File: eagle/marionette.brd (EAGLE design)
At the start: 112.4 x 152.7 mm, 45 parts, among them J2 SWD_CONNECTOR, J3 2X10FE, J4 2X10FE, J5 2X10FE, J6 2X10FE, J7 2X10FE, U1 USB3318, U2 NCP705, U3 XCL206B, X1 ABS25-32.768KHZ-6-T

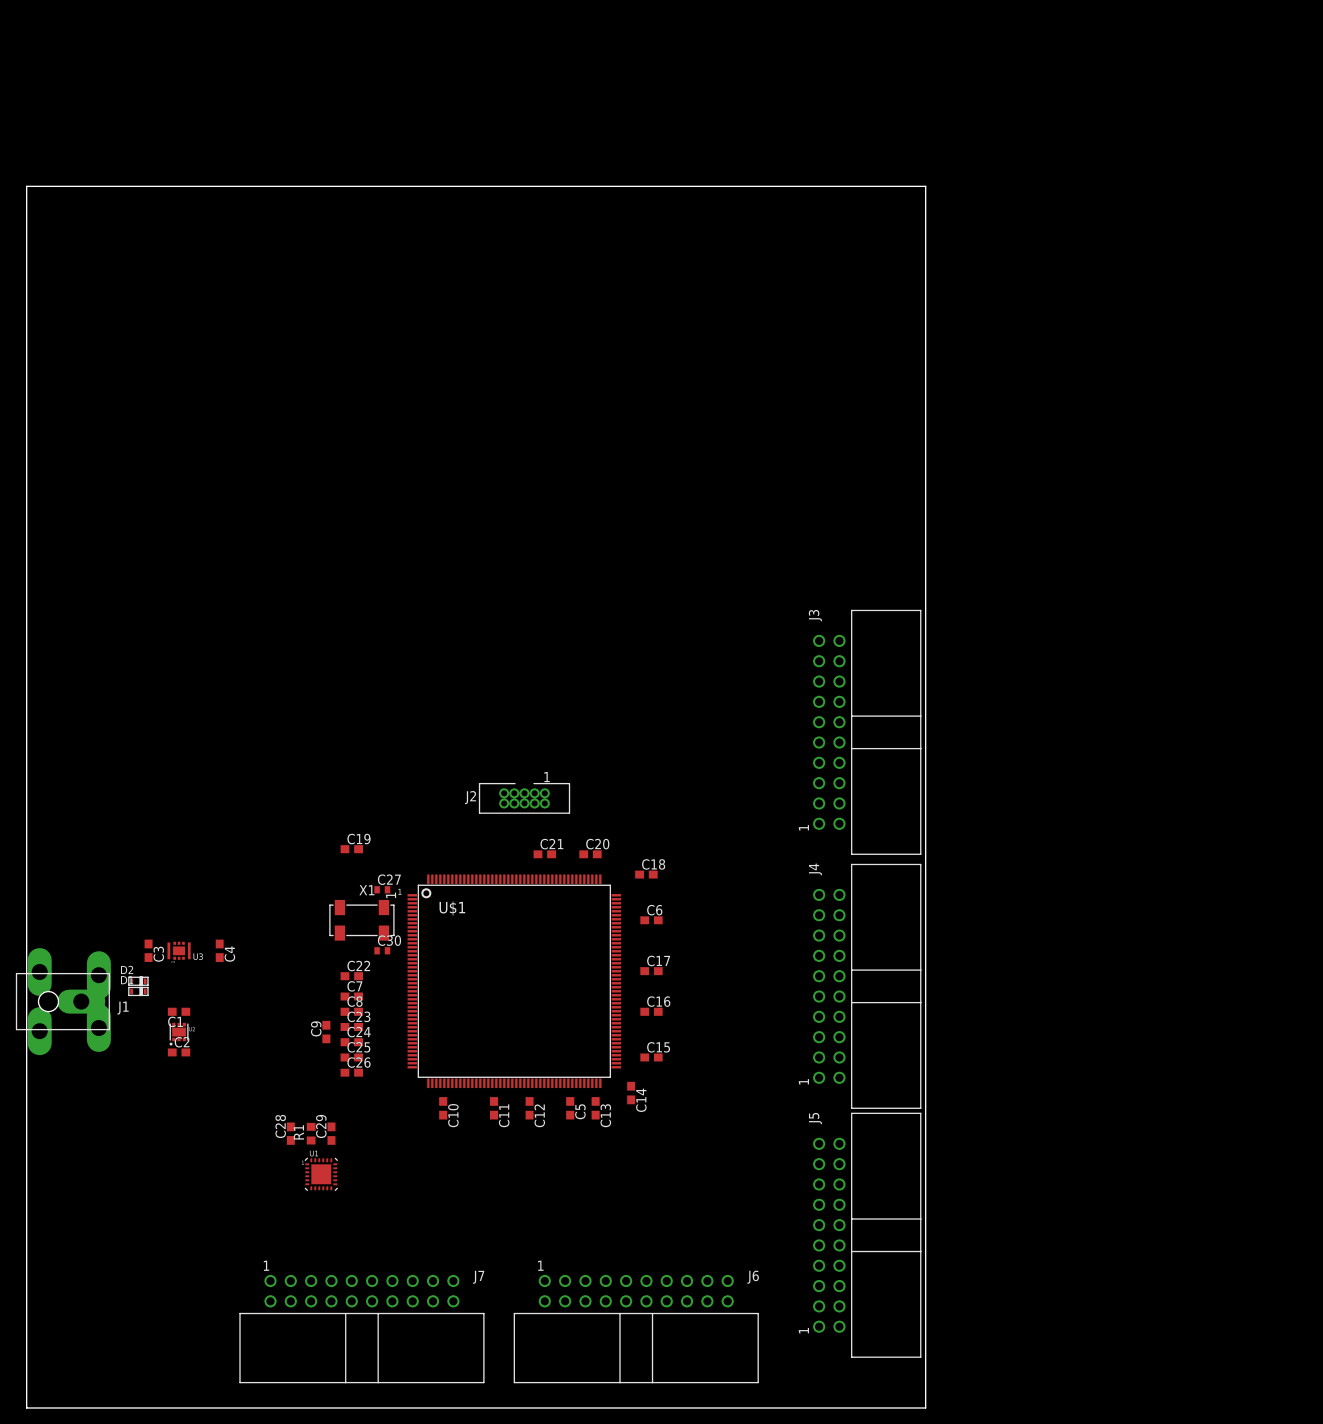
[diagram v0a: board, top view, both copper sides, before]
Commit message: Added connections to the EDGE CONNECTOR OF DEATH!!!!!!!!!!!!!
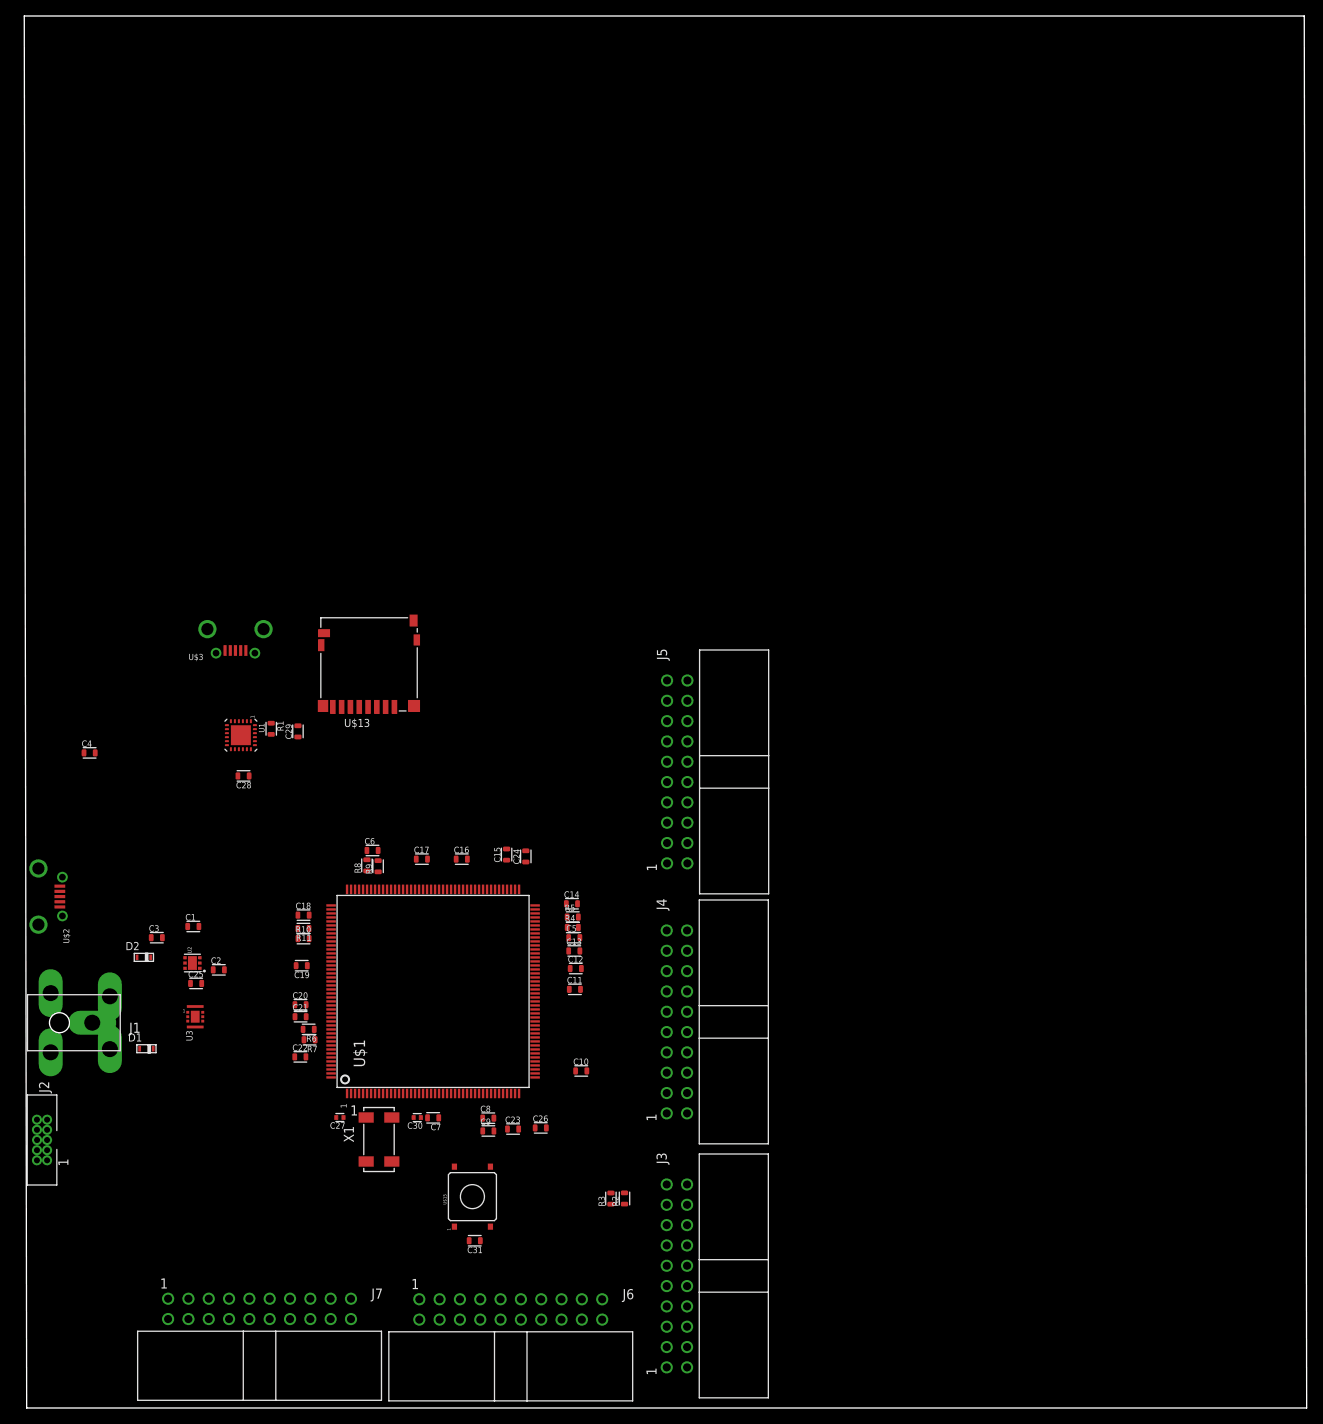
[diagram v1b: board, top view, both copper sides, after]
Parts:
- added C31: 100nF, 10V, rcl_custom:.0603-C
- added R10, R11, R2, R3, R4, R5, R6, R7, R8, R9: 4.7k, rcl_custom:.0603-C
- added U$13: CON_HIROSE_DM3D(MICROSD), con-microsd-hirose-dm3:HIROSE_DM3D(MICRO-SD)
- added U$15: PTS645, PTS645:SMT
- added U$2, U$3: ZX62D-B-5P8, con-hirose-microusb:ZX62D-B-5P8
- C1, C10, C11, C12, C13, C14, C15, C16, C17, C18, C19, C2, C20, C21, C22, C23, C24, C25, C26, C28, C29, C3, C4, C5, C6, C7, C8, C9: device CAPACITOR_SMT:C0603 -> rcl_custom:.0603-C
- C27, C30: device CAPACITOR_SMT:C0402 -> rcl_custom:.0402-C
- R1: device RESISTOR:R0603 -> rcl_custom:.0603-C
- moved J2 73.9 mm to (1.92, 33.5), turned to 90 degrees
- moved J3 70.6 mm to (81.3, 16.5)
- moved J5 61.0 mm to (81.3, 79.5)
- moved U1 55.8 mm to (26.8, 84.1), turned to 270 degrees
- moved R1 50.9 mm to (30.6, 84.9), turned to 270 degrees
- moved C29 50.5 mm to (33.9, 84.6)
- moved C28 45.1 mm to (27.1, 79.0), turned to 180 degrees
- moved C18 43.2 mm to (34.6, 61.6)
- moved C20 40.8 mm to (34.2, 50.4)
- moved C21 36.7 mm to (34.2, 48.9)
- moved C6 36.0 mm to (43.2, 69.7)
- moved C17 31.9 mm to (49.4, 68.6)
- moved C24 31.8 mm to (62.4, 69.0), turned to 90 degrees
- moved C15 31.2 mm to (60.0, 69.2), turned to 90 degrees
- moved C16 30.4 mm to (54.4, 68.6)
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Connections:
- new net CAN1_RX: J5.2, U$1.11
- new net CAN1_TX: J5.1, U$1.128
- new net DAC1: J4.20, U$1.50
- new net FS_DM: U$1.122, U$2.P2
- new net FS_DP: U$1.123, U$2.P3
- new net FS_ID: U$1.121, U$2.P4
- new net I2C1_SCL: R6.1, U$1.164
- new net I2C1_SDA: R7.1, U$1.165
- new net I2C2_SLC: J3.19
- new net I2C2_SMBA: J3.20, U$1.18
- new net I2C3_SCL: J6.2, R4.1, U$1.84
- new net I2C3_SDA: J6.1, R5.1, U$1.85
- new net N$10: U$3.P3, U1.6
- new net N$11: U$3.P4, U1.1
- new net OTG_VBUS: D2.P$1, U$1.120, U$2.P1
- new net PE0: J4.9, U$1.169
- new net PE1: J4.10, U$1.170
- new net PE10: J4.19, U$1.73
- new net PE11: J5.3, U$1.74
- new net PE12: J5.4, U$1.75
- new net PE13: J5.5, U$1.76
- new net PE14: J5.6, U$1.77
- new net PE15: J5.7, U$1.78
- new net PE2: J4.11, U$1.1
- new net PE3: J4.12, U$1.2
- new net PE4: J4.13, U$1.3
- new net PE5: J4.14, U$1.4
- new net PE6: J4.15, U$1.5
- new net PE7: J4.16, U$1.68
- new net PE8: J4.17, U$1.69
- new net PE9: J4.18, U$1.70
- new net PF11: J5.8, U$1.59
- new net PF12: J5.9, U$1.60
- new net PF13: J5.10, U$1.63
- new net PF14: J5.11, U$1.64
- new net PF15: J5.12, U$1.65
- new net PG0: J5.13, U$1.66
- new net PG1: J5.14, U$1.67
- new net PG10: J6.6, U$1.153
- new net PG11: J6.7, U$1.154
- new net PG12: J6.8, U$1.155
- new net PG13: J6.9, U$1.156
- new net PG14: J6.10, U$1.157
- new net PG15: J6.11, U$1.160
- new net PG2: J5.15, U$1.106
- new net PG3: J5.16, U$1.107
- new net PG4: J5.17, U$1.108
- new net PG5: J5.18, U$1.109
- new net PG6: J5.19, U$1.110
- new net PG7: J5.20, U$1.111
- new net PG8: J6.4, U$1.112
- new net PG9: J6.5, U$1.152
- new net UART4_RX: J4.2, U$1.41
- new net UART4_TX: J4.1, U$1.40
- net +3.3VDD: now also R10.2, R11.2, R2.2, R3.2, R4.2, R5.2, R6.2, R7.2, R8.2, R9.2, U$13.P4, U1.17
- net +3.3VDDA: no longer C23.1, C24.1, U$1.38
- net ADC1/2/3_IN11: now also J7.4
- net ADC1/2/3_IN13: now also J7.5
- net ADC1/2/3_IN2: now also J7.1
- net ADC1/2_IN14: now also J7.6
- net ADC1/2_IN15: now also J7.7
- net ADC1/2_IN6: now also J7.2
- net ADC1/2_IN7: now also J7.3
- net ADC3_IN14: now also J7.9
- net ADC3_IN15: now also J7.10
- net ADC3_IN4: now also J7.11
- net ADC3_IN5: now also J7.12
- net ADC3_IN6: now also J7.13
- net ADC3_IN7: now also J7.14
- net ADC3_IN8: now also J7.15, J7.8
- net GND: now also C29.2, C31.2, U$13.G1, U$13.G2, U$13.G3, U$13.G4, U$13.P6, U$15.1, U$15.2, U$2.P$1, U$2.P$2, U$2.P$3, U$2.P$4, U$2.P5, U$3.P$1, U$3.P$2, U$3.P$3, U$3.P$4, U$3.P5; no longer J3.20, J4.20, J5.20, J6.20, J7.20
- net I2C2_SCL: now also R3.1
- net I2C2_SDA: now also J3.18, R2.1
- net I2C3_SMBA: now also J6.3, U$1.86; no longer U$1.18
- net N$12: no longer C29.2
- net N$13: now also C31.1, U$1.31, U$15.3, U$15.4; no longer U$1.122
- net N$14: now also C23.1, C24.1, U$1.38; no longer U$1.123
- net N$2: now also U$3.P1, U1.2; no longer U$1.120
- net N$6: now also U$3.P2, U1.5; no longer U$1.121
- net PA15: now also J3.5
- net PB14: now also J3.7
- net PB4: now also J3.6
- net PC15: now also J3.8
- net PD0: now also J3.9
- net PD1: now also J3.10
- net PD10: now also J4.3
- net PD11: now also J4.4
- net PD12: now also J4.5
- net PD13: now also J4.6
- net PD14: now also J4.7
- net PD15: now also J4.8
- net PD3: now also J3.11
- net PD4: now also J3.12
- net PD5: now also J3.13
- net PD6: now also J3.14
- net PD7: now also J3.15
- net PD8: now also J3.16
- net PD9: now also J3.17
- net PH10: now also J6.16
- net PH11: now also J6.17
- net PH12: now also J6.18
- net PH14: now also J6.19
- net PH15: now also J6.20
- net PH2: now also J6.12
- net PH3: now also J6.13
- net PH5: now also J6.14
- net PH6: now also J6.15
- net PI4: now also J7.16
- net PI5: now also J7.17
- net PI6: now also J7.18
- net PI7: now also J7.19
- net PI8: now also J7.20
- net SDIO_CK: now also U$13.P5
- net SDIO_CMD: now also U$13.P3
- net SDIO_D0: now also R8.1, U$13.P7
- net SDIO_D1: now also U$13.P8
- net SDIO_D2: now also R11.1, U$13.P1
- net SDIO_D3: now also R10.1, R9.1, U$13.P2
- net SPI2_MISO: now also J3.3
- net SPI2_MOSI: now also J3.4
- net SPI2_NSS: now also J3.1
- net SPI2_SCK: now also J3.2
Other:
- board size 112.4 x 152.7 mm -> 160.3 x 174 mm
